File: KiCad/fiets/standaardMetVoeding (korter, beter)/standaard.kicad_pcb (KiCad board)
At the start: 2 copper layers, 92.7 x 69.3 mm, 24 parts, among them J1 Conn_01x04_Female, J2 R pinnen RGB strips, J3 282837-4, J4 282841-2, J5 12V DC, SW1 ENABLE, SW2 BOOT, U1 ESP32-WROOM-32E_(16MB)

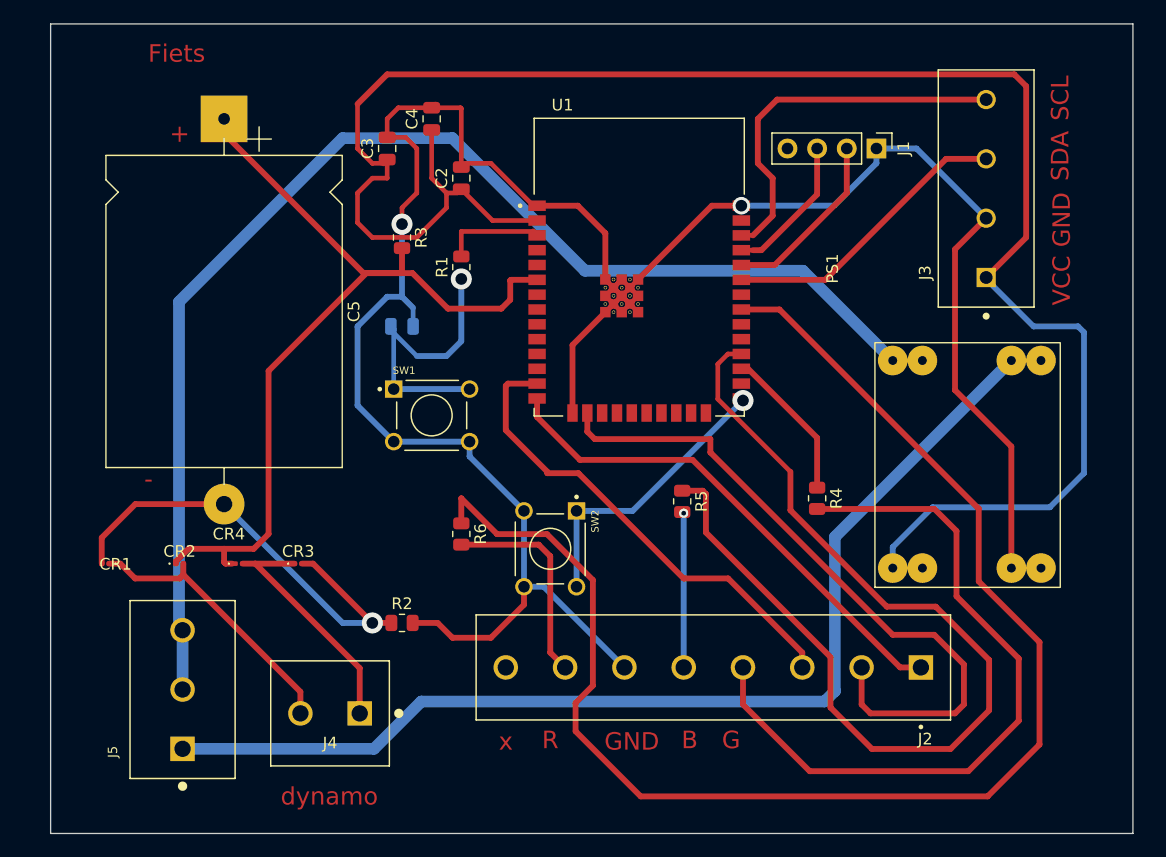
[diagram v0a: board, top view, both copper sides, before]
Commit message: aanpassingen
aanpass kicad fiets
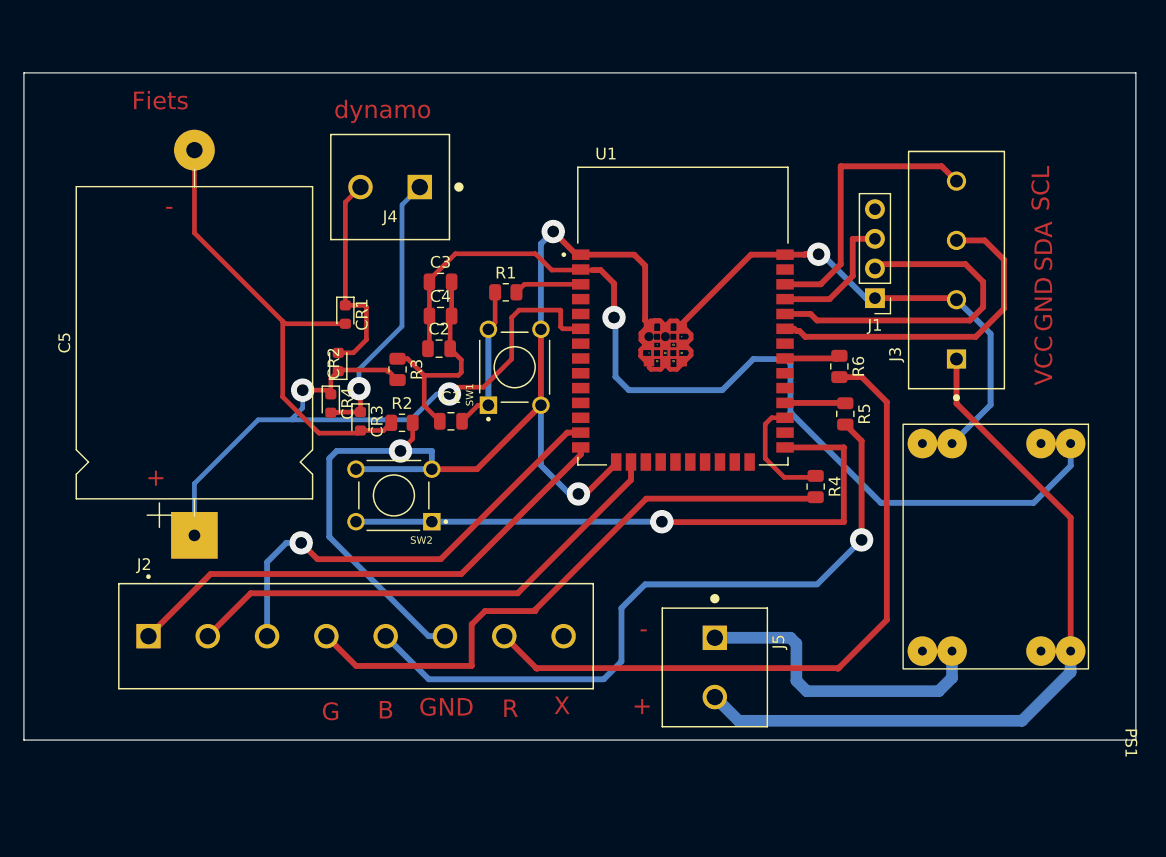
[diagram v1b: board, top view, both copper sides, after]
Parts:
- C1: moved to F.Cu
- CR1, CR2, CR3, CR4: footprint Diode_SMD:D_0201_0603Metric -> Diode_SMD:D_0603_1608Metric
- J5: value 12V DC -> 282841-2; footprint libraries:TE_282841-3 -> libraries:TE_282841-2
- moved J5 45.6 mm to (179.2, 77.5), turned to -90 degrees
- moved J4 45.4 mm to (151.4, 36.3)
- moved C5 35.8 mm to (134.6, 66.2), turned to 90 degrees
- moved R6 35.4 mm to (189.9, 51.7)
- moved J2 30.7 mm to (148.5, 74.8), turned to 0 degrees
- moved CR1 29.6 mm to (147.5, 47.2), turned to -90 degrees
- moved CR2 22.0 mm to (146.9, 51.3), turned to 90 degrees
- moved R2 17.1 mm to (152.4, 56.5)
- moved C4 16.9 mm to (155.7, 47.4), turned to 0 degrees
- moved R5 15.9 mm to (190.4, 55.8)
- moved CR4 15.8 mm to (146.3, 54.9), turned to -90 degrees
- moved C2 14.7 mm to (155.6, 50.2), turned to 0 degrees
- moved SW2 14.2 mm to (151.7, 62.7), turned to 180 degrees
- moved CR3 13.3 mm to (148.8, 56.4), turned to -90 degrees
- moved J1 12.8 mm to (192.9, 45.8), turned to 180 degrees
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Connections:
- J1 pad 4: +3V3 -> Net-(C2-Pad1)
- J3 pad 1: Net-(C2-Pad1) -> Net-(J3-Pad1)
- J5 pad 2: Net-(J5-Pad2) -> Net-(J3-Pad1)
- PS1 pad 1a: Net-(J5-Pad2) -> Net-(J3-Pad1)
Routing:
- net Net-(R6-Pad1): track 126.0 -> 4.75 mm
- net Net-(J5-Pad2): track 108.2 -> 0.00 mm
- net Net-(R5-Pad1): track 85.4 -> 5.17 mm
- net Net-(C2-Pad1): track 159.0 -> 82.5 mm, vias 0 -> 1
- net Net-(J5-Pad1): track 92.5 -> 26.8 mm
- net Net-(J3-Pad1): track 0.00 -> 63.9 mm
- net Net-(J2-Pad5): track 13.2 -> 60.6 mm
- net Net-(J2-Pad7): track 18.1 -> 59.6 mm
- net Net-(SW2-Pad1): track 24.7 -> 53.4 mm
- net GND: track 215.6 -> 195.2 mm, vias 2 -> 4
- net Net-(C5-Pad1): track 78.5 -> 60.8 mm, vias 0 -> 2
- net Net-(J2-Pad2): track 58.8 -> 43.3 mm
- net Net-(J1-Pad2): track 15.4 -> 29.9 mm
- net Net-(C1-Pad2): track 25.1 -> 12.7 mm, vias 1 -> 0
- net Net-(J2-Pad4): track 62.1 -> 51.1 mm
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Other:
- board size 92.7 x 69.3 mm -> 95.2 x 57.1 mm
- board text added: "X"
- board text removed: "x"
